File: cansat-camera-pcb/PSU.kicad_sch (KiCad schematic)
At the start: 6 parts, among them U1 AP2112K-3.3, U2 AP2112K-3.3

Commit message: send to production
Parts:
- U1, U2: footprint Package_TO_SOT_SMD:SOT-23-5_HandSoldering -> gaia-camera-footprints:SOT-23-5
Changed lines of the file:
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@@
 			)
 		)
-		(property "Footprint" "Package_TO_SOT_SMD:SOT-23-5_HandSoldering"
+		(property "Footprint" "gaia-camera-footprints:SOT-23-5"
 			(at 137.16 61.595 0)
 			(effects
@@
 			)
 		)
-		(property "Footprint" "Package_TO_SOT_SMD:SOT-23-5_HandSoldering"
+		(property "Footprint" "gaia-camera-footprints:SOT-23-5"
 			(at 73.66 61.595 0)
 			(effects

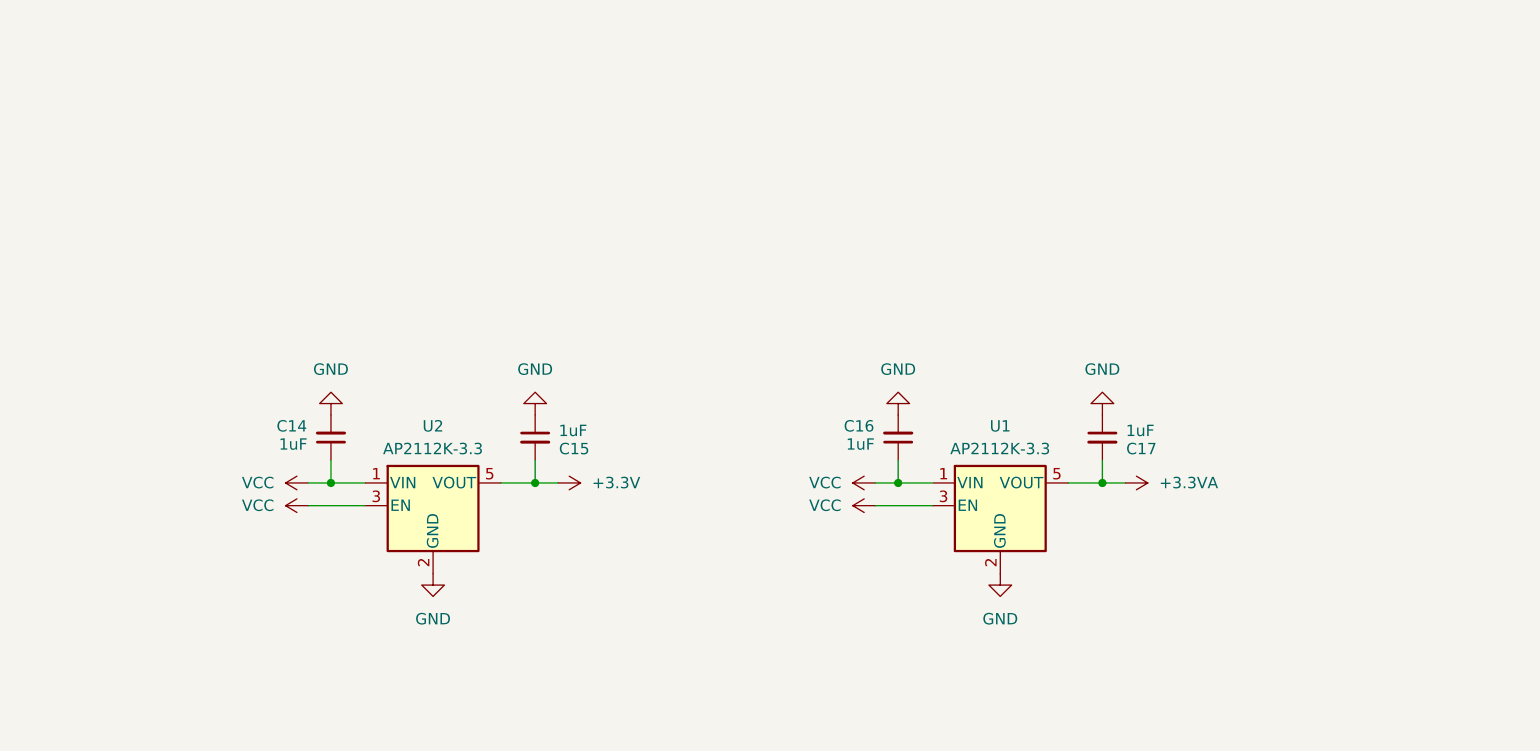
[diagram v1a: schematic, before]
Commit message: milan eszi a havat(unicummal)  (jonas is zabalja)
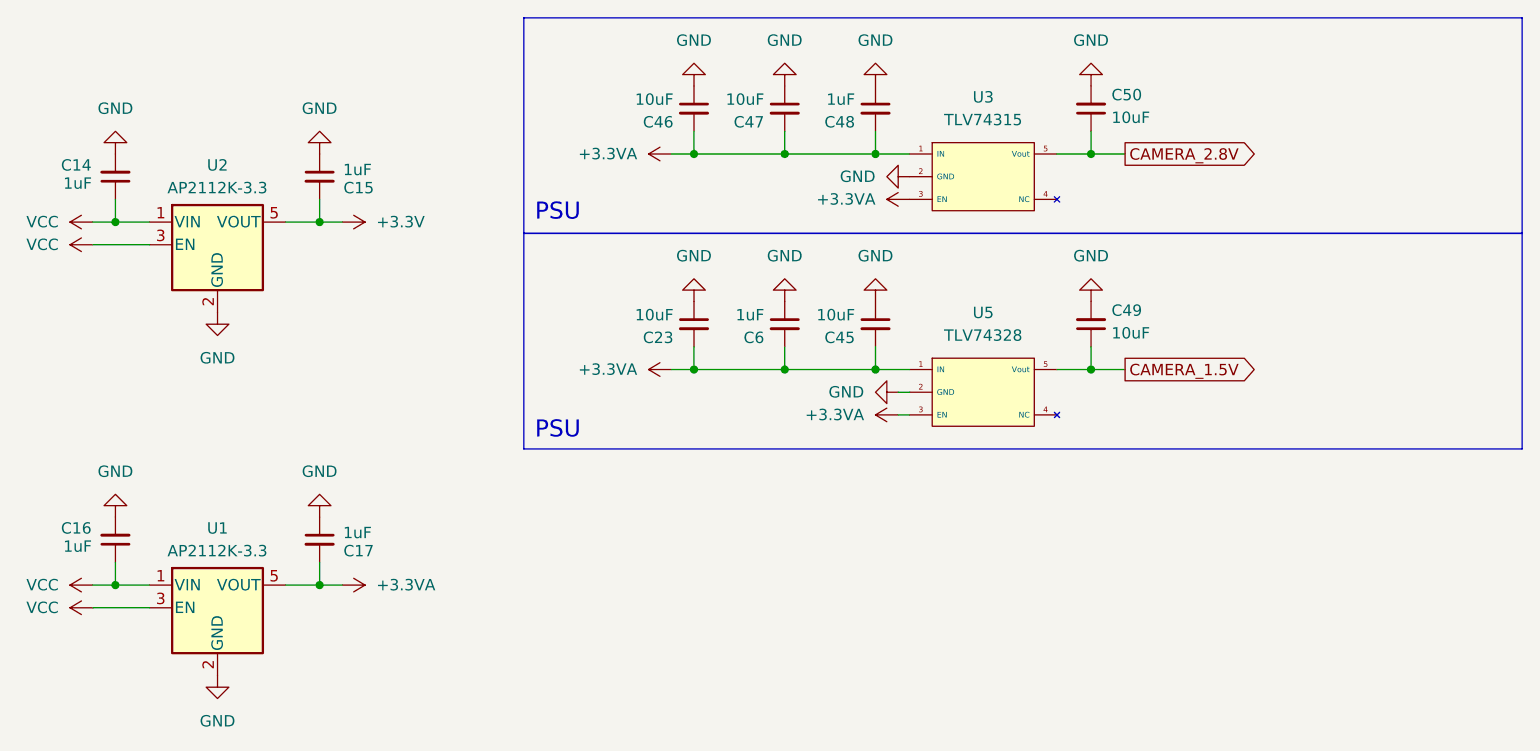
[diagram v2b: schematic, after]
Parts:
- added C23, C45, C46, C47, C49, C50: 10uF, Capacitor_SMD:C_0603_1608Metric, symbol Device:C_Small
- added C48, C6: 1uF, Capacitor_SMD:C_0603_1608Metric, symbol Device:C_Small
- added U3: TLV74315, gaia-camera-footprints:SOT-23-5, symbol gaia-camera-symbols:TLV74315
- added U5: TLV74328, gaia-camera-footprints:SOT-23-5, symbol gaia-camera-symbols:TLV74315
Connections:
- net +3.3VA: now also C23.2, C45.2, C46.2, C47.2, C48.2, C6.2, U3.1 (IN), U3.3 (EN), U5.1 (IN), U5.3 (EN)
- net GND: now also C23.1, C45.1, C46.1, C47.1, C48.1, C49.2, C50.2, C6.1, U3.2 (GND), U5.2 (GND)
- new net CAMERA_1.5V: C49.1, U5.5 (Vout)
- new net CAMERA_2.8V: C50.1, U3.5 (Vout)
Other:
- note added: "PSU"
- moved on the sheet: C14, C15, C16, C17, U1, U2
